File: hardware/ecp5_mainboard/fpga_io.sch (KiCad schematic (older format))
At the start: 74 parts, among them J10 UART, J11 FLASH, J12 JTAG, J5 EXT0, J6 EXT1, J7 EXT2, J9 PMOD_01, Q9 BSH111BKR, SW6 SW_Push, U15 ECP5UM5G_85_CABGA756, U26 XL_XO_LVDS, U27 W25Q

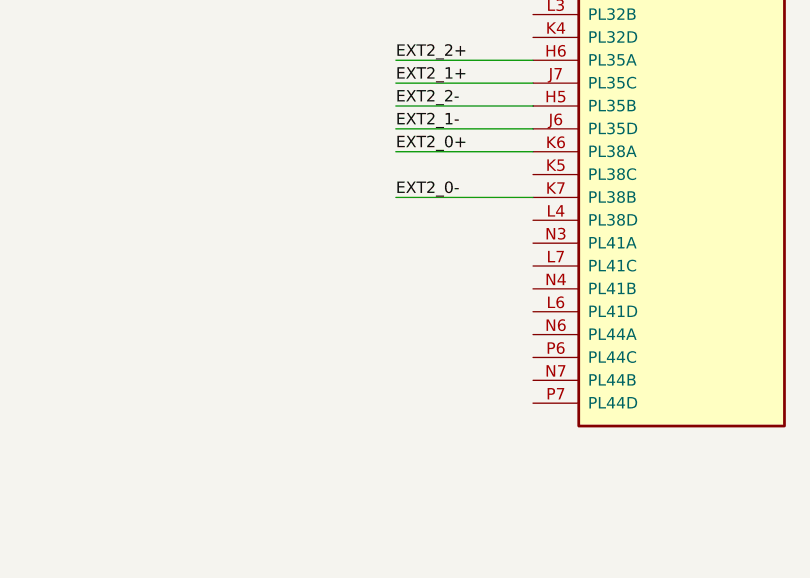
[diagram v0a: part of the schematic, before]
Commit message: hardware/mainboard: Switching from SATA to m.2 connector for second DCU
Signed-off-by: David Shah <dave@ds0.me>
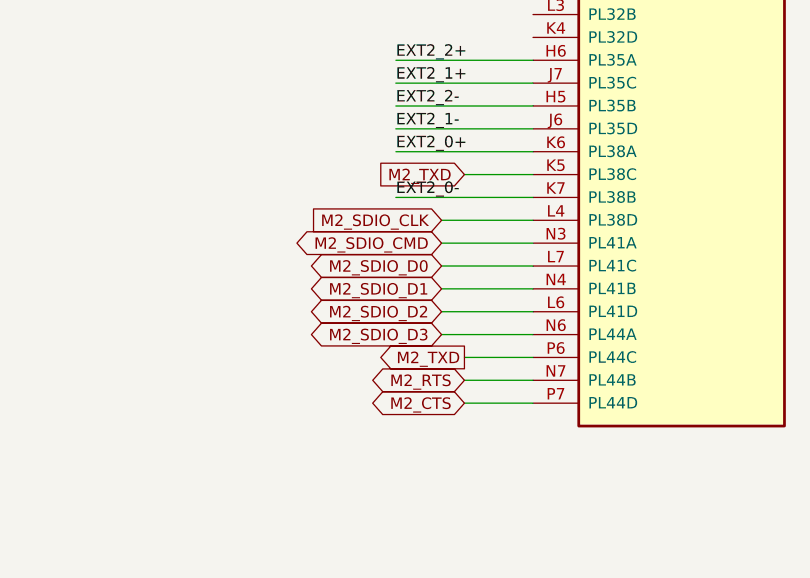
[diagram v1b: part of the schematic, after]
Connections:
- net M2_TXD: now reaches U15.K5 (PL38C)
- net M2_TXD: now also U15.P6 (PL44C)
- net M2_SDIO_CLK: now reaches U15.L4 (PL38D)
- net M2_SDIO_D2: now reaches U15.L6 (PL41D)
- net M2_SDIO_D0: now reaches U15.L7 (PL41C)
- net M2_SDIO_CMD: now reaches U15.N3 (PL41A)
- net M2_SDIO_D1: now reaches U15.N4 (PL41B)
- net M2_SDIO_D3: now reaches U15.N6 (PL44A)
- net M2_RTS: now reaches U15.N7 (PL44B)
- net M2_CTS: now reaches U15.P7 (PL44D)
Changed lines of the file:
@@
 Wire Bus Line
 	12350 2100 12550 2100
+Text GLabel 12150 13200 0    50   Input ~ 0
+M2_SDIO_CLK
+Text GLabel 12150 13300 0    50   BiDi ~ 0
+M2_SDIO_CMD
+Text GLabel 12150 13400 0    50   BiDi ~ 0
+M2_SDIO_D0
+Text GLabel 12150 13500 0    50   BiDi ~ 0
+M2_SDIO_D1
+Text GLabel 12150 13600 0    50   BiDi ~ 0
+M2_SDIO_D2
+Text GLabel 12150 13700 0    50   BiDi ~ 0
+M2_SDIO_D3
+Wire Wire Line
+	12150 13200 12550 13200
+Wire Wire Line
+	12150 13300 12550 13300
+Wire Wire Line
+	12150 13400 12550 13400
+Wire Wire Line
+	12150 13500 12550 13500
+Wire Wire Line
+	12150 13600 12550 13600
+Wire Wire Line
+	12150 13700 12550 13700
+Wire Wire Line
+	12550 13000 12250 13000
+Text GLabel 12250 13000 0    50   Input ~ 0
+M2_TXD
+Text GLabel 12250 13800 0    50   Output ~ 0
+M2_TXD
+Wire Wire Line
+	12250 13800 12550 13800
+Text GLabel 12250 13900 0    50   BiDi ~ 0
+M2_RTS
+Text GLabel 12250 14000 0    50   BiDi ~ 0
+M2_CTS
+Wire Wire Line
+	12250 13900 12550 13900
+Wire Wire Line
+	12550 14000 12250 14000
 $EndSCHEMATC

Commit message: hardware/mainboard: Add and place M.2 connector footprint
Signed-off-by: David Shah <davey1576@gmail.com>
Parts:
- U27: symbol pkl_memory:W25Q -> ecp5_mainboard-rescue:W25Q-pkl_memory
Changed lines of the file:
@@
 ~INIT
 $Comp
-L pkl_memory:W25Q U27
+L ecp5_mainboard-rescue:W25Q-pkl_memory U27
 U 1 1 60E46888
 P 20600 9650
+AR Path="/60E46888" Ref="U27"  Part="1"
+AR Path="/61FAF948/60E46888" Ref="U27"  Part="1"
 F 0 "U27" H 20600 10075 50  0000 C CNN
 F 1 "W25Q" H 20600 9984 50  0000 C CNN
